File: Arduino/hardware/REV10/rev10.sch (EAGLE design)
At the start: 46 parts, among them IC2 ATMEGA168-AU, Q1 32768Hz, U1 TC1185SMD

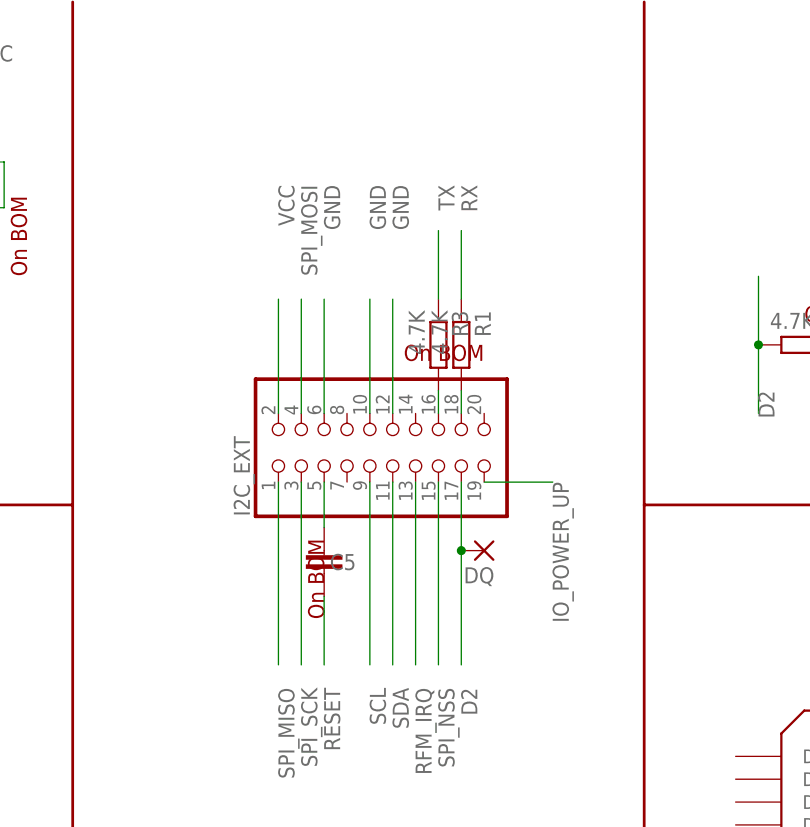
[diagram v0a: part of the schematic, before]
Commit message: rev 10 routed
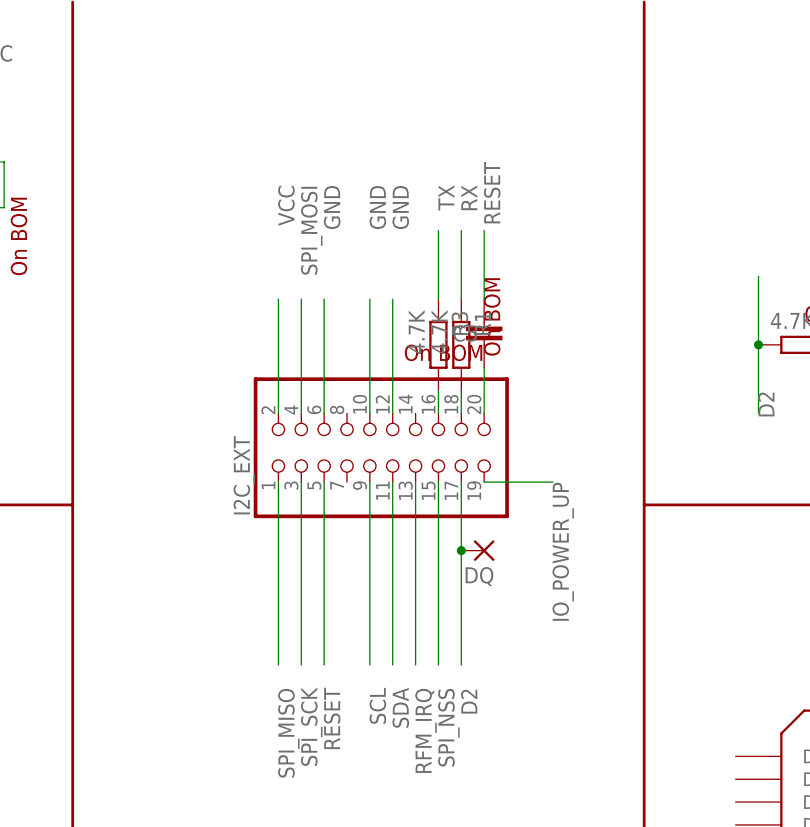
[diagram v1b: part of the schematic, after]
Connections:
- net N$26: now also I2C_EXT.20; no longer I2C_EXT.5
- net RESET: now also I2C_EXT.5
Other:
- moved on the sheet: C5
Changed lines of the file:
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@@
 <text x="307.34" y="177.8" size="1.778" layer="94" rot="R90">On BOM</text>
 <text x="45.72" y="175.26" size="1.778" layer="94" rot="R180">On BOM</text>
-<text x="121.92" y="195.58" size="1.778" layer="94" rot="R90">On BOM</text>
+<text x="139.7" y="233.68" size="1.778" layer="94" rot="R270">On BOM</text>
 <wire x1="325.12" y1="157.48" x2="325.12" y2="124.46" width="0.3048" layer="94"/>
 <wire x1="325.12" y1="124.46" x2="325.12" y2="83.82" width="0.3048" layer="94"/>
@@
 <instance part="R1" gate="G$1" x="137.16" y="226.06" rot="R270"/>
 <instance part="R3" gate="G$1" x="134.62" y="226.06" rot="R270"/>
-<instance part="C5" gate="G$1" x="121.92" y="200.66" smashed="yes" rot="R180">
-<attribute name="NAME" x="125.476" y="202.819" size="1.778" layer="95" rot="R180"/>
+<instance part="C5" gate="G$1" x="139.7" y="228.6" smashed="yes">
+<attribute name="NAME" x="136.144" y="226.441" size="1.778" layer="95"/>
 </instance>
 <instance part="JP1" gate="A" x="271.78" y="106.68" smashed="yes">
@@
 <segment>
 <pinref part="C5" gate="G$1" pin="1"/>
-<wire x1="121.92" y1="198.12" x2="121.92" y2="190.5" width="0.1524" layer="91"/>
+<wire x1="139.7" y1="231.14" x2="139.7" y2="238.76" width="0.1524" layer="91"/>
+<label x="139.7" y="246.38" size="1.778" layer="95" rot="R270"/>
+</segment>
+<segment>
+<wire x1="121.92" y1="190.5" x2="121.92" y2="210.82" width="0.1524" layer="91"/>
 <label x="121.92" y="187.96" size="1.778" layer="95" rot="R270"/>
+<pinref part="I2C_EXT" gate="A" pin="5"/>
 </segment>
 </net>
@@
 <net name="N$26" class="0">
 <segment>
-<wire x1="121.92" y1="210.82" x2="121.92" y2="205.74" width="0.1524" layer="91"/>
+<pinref part="I2C_EXT" gate="A" pin="20"/>
 <pinref part="C5" gate="G$1" pin="2"/>
-<pinref part="I2C_EXT" gate="A" pin="5"/>
-</segment>
-</net>
+<wire x1="139.7" y1="218.44" x2="139.7" y2="223.52" width="0.1524" layer="91"/>
+</segment>
+</net>

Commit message: fixed rev10 transistor
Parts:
- T1: device transistor:-NPN-SOT23-EBC -> transistor:MMBTH24LT1-NPN-SOT23-BEC
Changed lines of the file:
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@@
 <?xml version="1.0" encoding="utf-8"?>
 <!DOCTYPE eagle SYSTEM "eagle.dtd">
-<eagle version="7.4.0">
+<eagle version="7.5.0">
 <drawing>
 <settings>
@@
 <grid distance="0.1" unitdist="inch" unit="inch" style="lines" multiple="1" display="no" altdistance="0.01" altunitdist="inch" altunit="inch"/>
 <layers>
-<layer number="1" name="Top" color="4" fill="1" visible="no" active="no"/>
-<layer number="16" name="Bottom" color="1" fill="1" visible="no" active="no"/>
-<layer number="17" name="Pads" color="2" fill="1" visible="no" active="no"/>
-<layer number="18" name="Vias" color="2" fill="1" visible="no" active="no"/>
-<layer number="19" name="Unrouted" color="6" fill="1" visible="no" active="no"/>
-<layer number="20" name="Dimension" color="15" fill="1" visible="no" active="no"/>
-<layer number="21" name="tPlace" color="7" fill="1" visible="no" active="no"/>
-<layer number="22" name="bPlace" color="7" fill="1" visible="no" active="no"/>
-<layer number="23" name="tOrigins" color="15" fill="1" visible="no" active="no"/>
-<layer number="24" name="bOrigins" color="15" fill="1" visible="no" active="no"/>
-<layer number="25" name="tNames" color="7" fill="1" visible="no" active="no"/>
-<layer number="26" name="bNames" color="7" fill="1" visible="no" active="no"/>
-<layer number="27" name="tValues" color="7" fill="1" visible="no" active="no"/>
-<layer number="28" name="bValues" color="7" fill="1" visible="no" active="no"/>
+<layer number="1" name="Top" color="4" fill="1" visible="yes" active="no"/>
+<layer number="16" name="Bottom" color="1" fill="1" visible="yes" active="no"/>
+<layer number="17" name="Pads" color="2" fill="1" visible="yes" active="no"/>
+<layer number="18" name="Vias" color="2" fill="1" visible="yes" active="no"/>
+<layer number="19" name="Unrouted" color="6" fill="1" visible="yes" active="no"/>
+<layer number="20" name="Dimension" color="15" fill="1" visible="yes" active="no"/>
+<layer number="21" name="tPlace" color="7" fill="1" visible="yes" active="no"/>
+<layer number="22" name="bPlace" color="7" fill="1" visible="yes" active="no"/>
+<layer number="23" name="tOrigins" color="15" fill="1" visible="yes" active="no"/>
+<layer number="24" name="bOrigins" color="15" fill="1" visible="yes" active="no"/>
+<layer number="25" name="tNames" color="7" fill="1" visible="yes" active="no"/>
+<layer number="26" name="bNames" color="7" fill="1" visible="yes" active="no"/>
+<layer number="27" name="tValues" color="7" fill="1" visible="yes" active="no"/>
+<layer number="28" name="bValues" color="7" fill="1" visible="yes" active="no"/>
 <layer number="29" name="tStop" color="7" fill="3" visible="no" active="no"/>
 <layer number="30" name="bStop" color="7" fill="6" visible="no" active="no"/>
@@
 <layer number="35" name="tGlue" color="7" fill="4" visible="no" active="no"/>
 <layer number="36" name="bGlue" color="7" fill="5" visible="no" active="no"/>
-<layer number="37" name="tTest" color="7" fill="1" visible="no" active="no"/>
-<layer number="38" name="bTest" color="7" fill="1" visible="no" active="no"/>
+<layer number="37" name="tTest" color="7" fill="1" visible="yes" active="no"/>
+<layer number="38" name="bTest" color="7" fill="1" visible="yes" active="no"/>
 <layer number="39" name="tKeepout" color="4" fill="11" visible="no" active="no"/>
 <layer number="40" name="bKeepout" color="1" fill="11" visible="no" active="no"/>
@@
 <layer number="44" name="Drills" color="7" fill="1" visible="no" active="no"/>
 <layer number="45" name="Holes" color="7" fill="1" visible="no" active="no"/>
-<layer number="46" name="Milling" color="3" fill="1" visible="no" active="no"/>
-<layer number="47" name="Measures" color="7" fill="1" visible="no" active="no"/>
-<layer number="48" name="Document" color="7" fill="1" visible="no" active="no"/>
-<layer number="49" name="Reference" color="7" fill="1" visible="no" active="no"/>
-<layer number="50" name="dxf" color="7" fill="1" visible="no" active="no"/>
-<layer number="51" name="tDocu" color="7" fill="1" visible="no" active="no"/>
-<layer number="52" name="bDocu" color="7" fill="1" visible="no" active="no"/>
-<layer number="53" name="tGND_GNDA" color="7" fill="9" visible="no" active="no"/>
-<layer number="54" name="bGND_GNDA" color="1" fill="9" visible="no" active="no"/>
-<layer number="56" name="wert" color="7" fill="1" visible="no" active="no"/>
-<layer number="57" name="tCAD" color="7" fill="1" visible="no" active="no"/>
+<layer number="46" name="Milling" color="3" fill="1" visible="yes" active="no"/>
+<layer number="47" name="Measures" color="7" fill="1" visible="yes" active="no"/>
+<layer number="48" name="Document" color="7" fill="1" visible="yes" active="no"/>
+<layer number="49" name="Reference" color="7" fill="1" visible="yes" active="no"/>
+<layer number="50" name="dxf" color="7" fill="1" visible="yes" active="no"/>
+<layer number="51" name="tDocu" color="7" fill="1" visible="yes" active="no"/>
+<layer number="52" name="bDocu" color="7" fill="1" visible="yes" active="no"/>
+<layer number="53" name="tGND_GNDA" color="7" fill="9" visible="yes" active="no"/>
+<layer number="54" name="bGND_GNDA" color="1" fill="9" visible="yes" active="no"/>
+<layer number="56" name="wert" color="7" fill="1" visible="yes" active="no"/>
+<layer number="57" name="tCAD" color="7" fill="1" visible="yes" active="no"/>
 <layer number="90" name="Modules" color="5" fill="1" visible="yes" active="yes"/>
 <layer number="91" name="Nets" color="2" fill="1" visible="yes" active="yes"/>
@@
 <part name="R11" library="resistor" deviceset="R-EU_" device="R0603" value="470R"/>
 <part name="LED1" library="led" deviceset="LED" device="CHIP-LED0603"/>
-<part name="T1" library="transistor" deviceset="*-NPN-" device="SOT23-EBC"/>
+<part name="T1" library="transistor" deviceset="*-NPN-" device="SOT23-BEC" technology="MMBTH24LT1"/>
 <part name="R13" library="resistor" deviceset="R-EU_" device="R0603" value="1K"/>
 <part name="R14" library="resistor" deviceset="R-EU_" device="R0603" value="10K"/>
